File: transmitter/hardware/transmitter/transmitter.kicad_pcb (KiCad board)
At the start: 2 copper layers, 18 parts, among them J1 SOIL, J2 Conn_01x05, SW1 SW_SPST, SW2 SW_SPST, U1 NodeMCU_1.0_(ESP-12E), U2 MCP1700-3302E_SOT89, U3 CD4051B

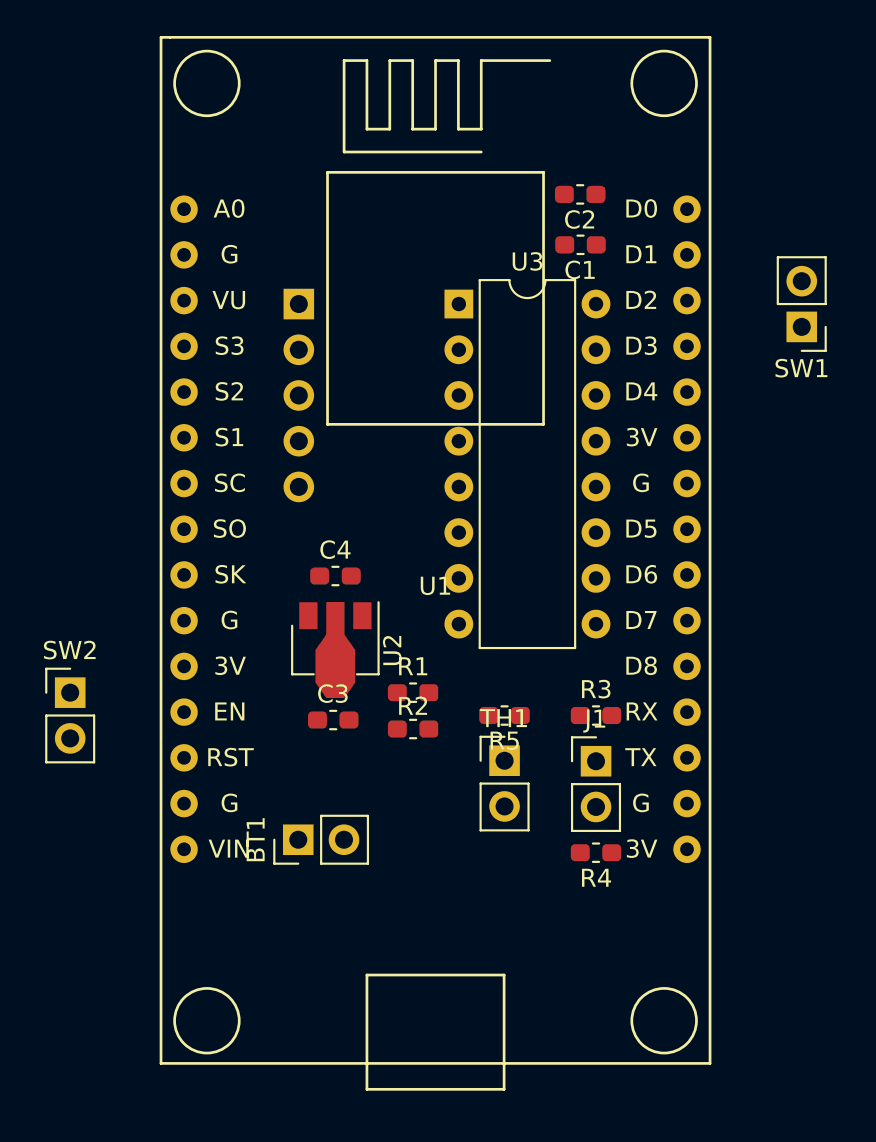
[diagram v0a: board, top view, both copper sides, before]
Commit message: Layout
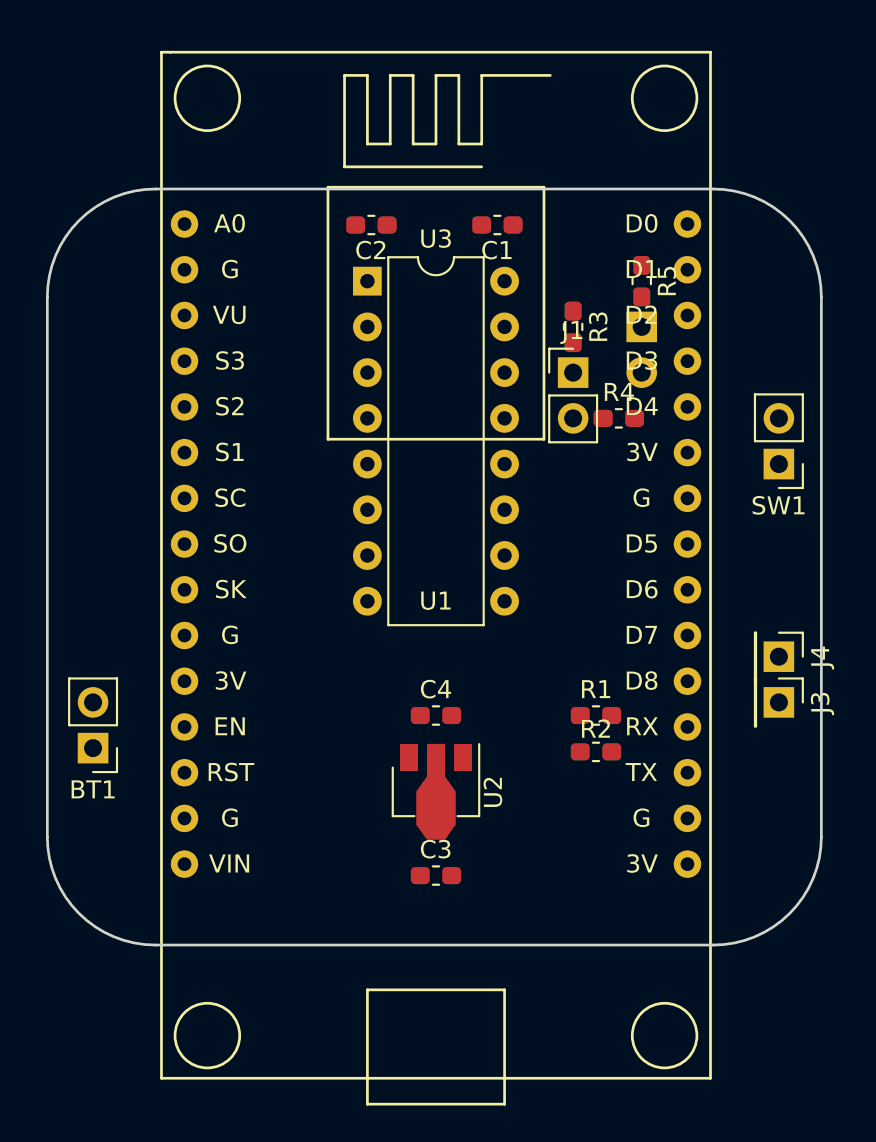
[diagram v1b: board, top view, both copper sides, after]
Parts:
- removed J2: Conn_01x05, Connector_PinHeader_2.54mm:PinHeader_1x05_P2.54mm_Vertical
- removed SW2: SW_SPST, Connector_PinHeader_2.54mm:PinHeader_1x02_P2.54mm_Vertical
- added J3: USB_UART_OFF, Connector_PinHeader_2.54mm:PinHeader_1x01_P2.54mm_Vertical, F.Cu at (167.6, 94.5)
- added J4: USB_UART_ON, Connector_PinHeader_2.54mm:PinHeader_1x01_P2.54mm_Vertical, F.Cu at (167.6, 92.0)
- TH1: moved to B.Cu
- moved R5 25.3 mm to (160.0, 71.1), turned to 270 degrees
- moved TH1 25.3 mm to (160.0, 73.7), turned to 180 degrees
- moved R4 24.2 mm to (158.8, 78.7), turned to 0 degrees
- moved J1 21.6 mm to (156.2, 76.2)
- moved R3 21.6 mm to (156.2, 73.7), turned to 270 degrees
- moved BT1 12.5 mm to (129.5, 97.1), turned to 180 degrees
- moved C2 11.7 mm to (145.0, 68.0)
- moved C3 10.4 mm to (148.6, 104.1)
- moved R1 10.2 mm to (157.5, 95.2)
- moved R2 10.2 mm to (157.5, 97.3)
- moved U2 9.66 mm to (148.6, 99.1)
- moved C4 9.55 mm to (148.6, 95.2)
- moved SW1 7.73 mm to (167.6, 81.3)
- moved U3 5.24 mm to (144.8, 71.1)
- moved C1 4.75 mm to (152.0, 68.0)
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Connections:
- U1 pad 10: Net-(U1-Pad10) -> (no net)
- U1 pad 12: Net-(U1-Pad12) -> (no net)
- U1 pad 15: /USB_UART_PWR -> (no net)
- U1 pad 16: Net-(U1-Pad16) -> (no net)
- U1 pad 17: Net-(U1-Pad17) -> (no net)
- U1 pad 18: Net-(U1-Pad18) -> (no net)
- U1 pad 19: Net-(U1-Pad19) -> (no net)
- U1 pad 2: Net-(U1-Pad2) -> (no net)
- U1 pad 20: Net-(U1-Pad20) -> (no net)
- U1 pad 24: Net-(U1-Pad24) -> (no net)
- U1 pad 25: Net-(U1-Pad25) -> (no net)
- U1 pad 26: Net-(U1-Pad26) -> (no net)
- U1 pad 27: Net-(U1-Pad27) -> (no net)
- U1 pad 28: Net-(U1-Pad28) -> (no net)
- U1 pad 3: Net-(U1-Pad3) -> (no net)
- U1 pad 4: Net-(U1-Pad4) -> (no net)
- U1 pad 5: Net-(U1-Pad5) -> (no net)
- U1 pad 6: Net-(U1-Pad6) -> (no net)
- U1 pad 7: Net-(U1-Pad7) -> (no net)
- U1 pad 8: Net-(U1-Pad8) -> (no net)
- U1 pad 9: Net-(U1-Pad9) -> (no net)
- U3 pad 1: Net-(J2-Pad2) -> (no net)
- U3 pad 12: Net-(J2-Pad1) -> (no net)
- U3 pad 2: Net-(J2-Pad4) -> (no net)
- U3 pad 4: Net-(J2-Pad5) -> (no net)
- U3 pad 5: Net-(J2-Pad3) -> (no net)
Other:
- board outline added: 43 x 42 mm

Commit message: All connected
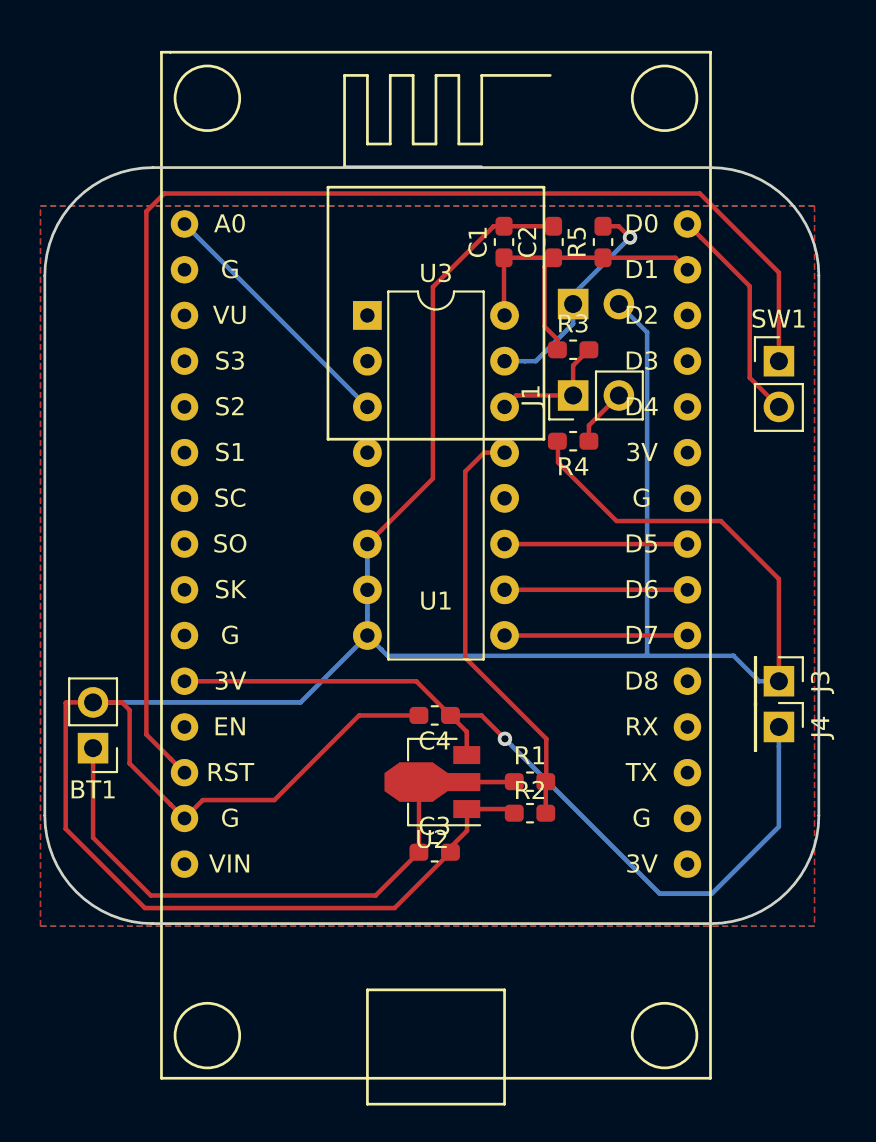
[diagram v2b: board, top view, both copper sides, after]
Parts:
- moved C2 10.2 mm to (155.1, 68.9), turned to 90 degrees
- moved SW1 5.72 mm to (167.6, 75.6), turned to 0 degrees
- moved R1 5.19 mm to (153.8, 98.9)
- moved R2 5.00 mm to (153.8, 100.7)
- moved TH1 4.02 mm to (156.2, 72.4), turned to 270 degrees
- moved J4 3.91 mm to (167.6, 95.9)
- moved R5 3.06 mm to (157.9, 68.9), turned to 90 degrees
- moved R4 2.84 mm to (156.2, 80.0), turned to 180 degrees
- moved U3 1.91 mm to (144.8, 73.0)
- moved C3 1.30 mm to (148.5, 102.8)
- moved R3 1.27 mm to (156.2, 74.9), turned to 0 degrees
- moved J1 1.27 mm to (156.2, 77.5), turned to 90 degrees
- moved J3 1.17 mm to (167.6, 93.3)
- moved C1 1.01 mm to (152.4, 68.9), turned to 90 degrees
- moved U2 0.26 mm to (148.8, 98.9), turned to 180 degrees
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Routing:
- net GND: track 0.00 -> 175.1 mm
- net RESET: track 0.00 -> 74.4 mm
- net 3V3: track 0.00 -> 47.6 mm, vias 0 -> 1
- net /BATT: track 0.00 -> 36.2 mm
- net BATT_SENSE: track 0.00 -> 23.5 mm
- net SENSE_PWR: track 0.00 -> 19.3 mm
- net A0: track 0.00 -> 14.4 mm
- net TEMP_SENSE: track 0.00 -> 12.5 mm, vias 0 -> 1
- net Net-(SW1-Pad2): track 0.00 -> 12.3 mm
- net Net-(U1-Pad23): track 0.00 -> 10.2 mm
- net Net-(U1-Pad22): track 0.00 -> 10.2 mm
- net Net-(U1-Pad21): track 0.00 -> 10.2 mm
- net SOIL_SENSE: track 0.00 -> 6.98 mm
- net Net-(J1-Pad2): track 0.00 -> 3.23 mm
- added copper zone on B.Cu, net GND
- added copper zone on F.Cu, net GND

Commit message: Power traces
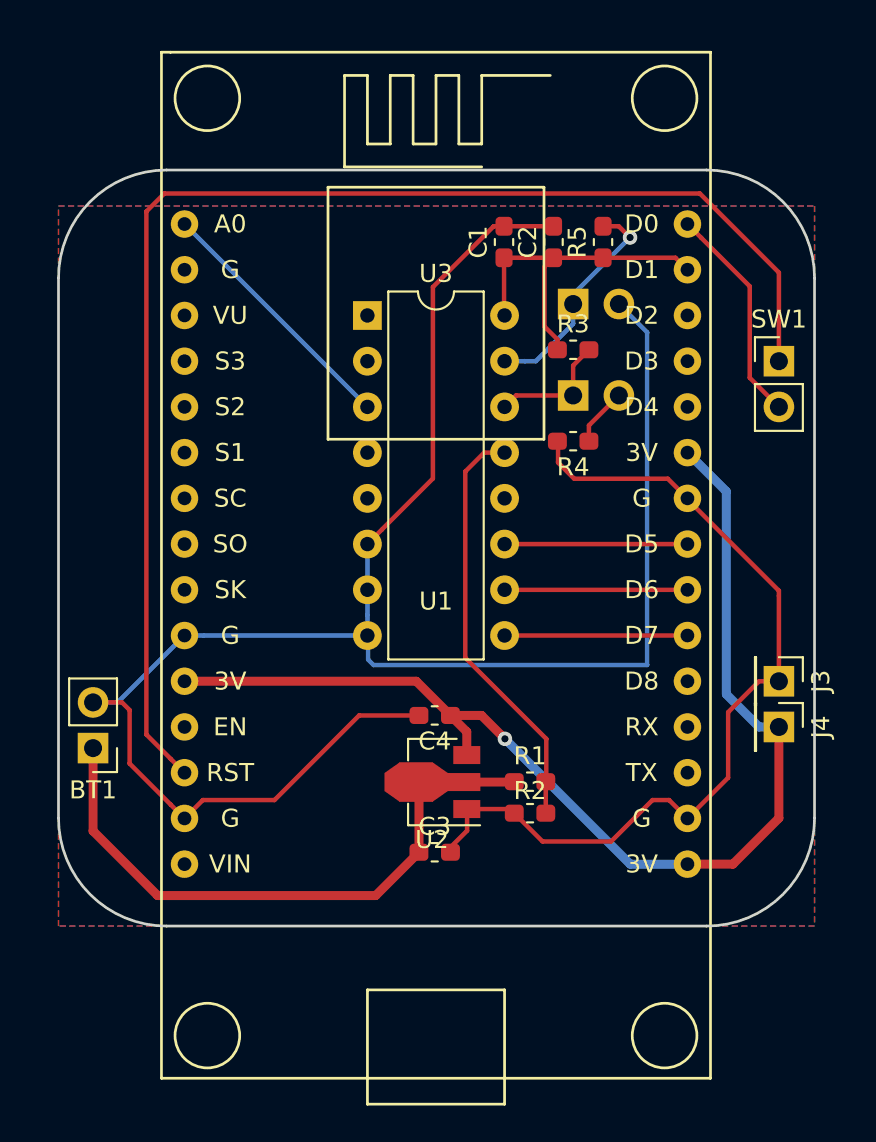
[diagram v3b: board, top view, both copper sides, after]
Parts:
- J1: moved to B.Cu
- turned J1 to 270 degrees
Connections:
- U1 pad 10: (no net) -> GND
- U1 pad 16: (no net) -> 3V3
- U1 pad 17: (no net) -> GND
- U1 pad 24: (no net) -> GND
- U1 pad 25: (no net) -> 3V3
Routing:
- net GND: track 175.1 -> 157.3 mm
- net 3V3: track 47.6 -> 63.9 mm
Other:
- board size 43 x 42 mm -> 42 x 42 mm
- net class BATT added: clearance 0.25, trace_width 0.5, via_dia 0.8, via_drill 0.4
